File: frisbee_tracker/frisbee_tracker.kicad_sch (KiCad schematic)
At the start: 18 parts, among them IC1 NRF54L05-QFAA-R7, J1 UJC-H-G-SMT-2-P6-TR, U1 AP2210N-3.3TRG1, U2 BQ24072RGTT, U3 BMI323

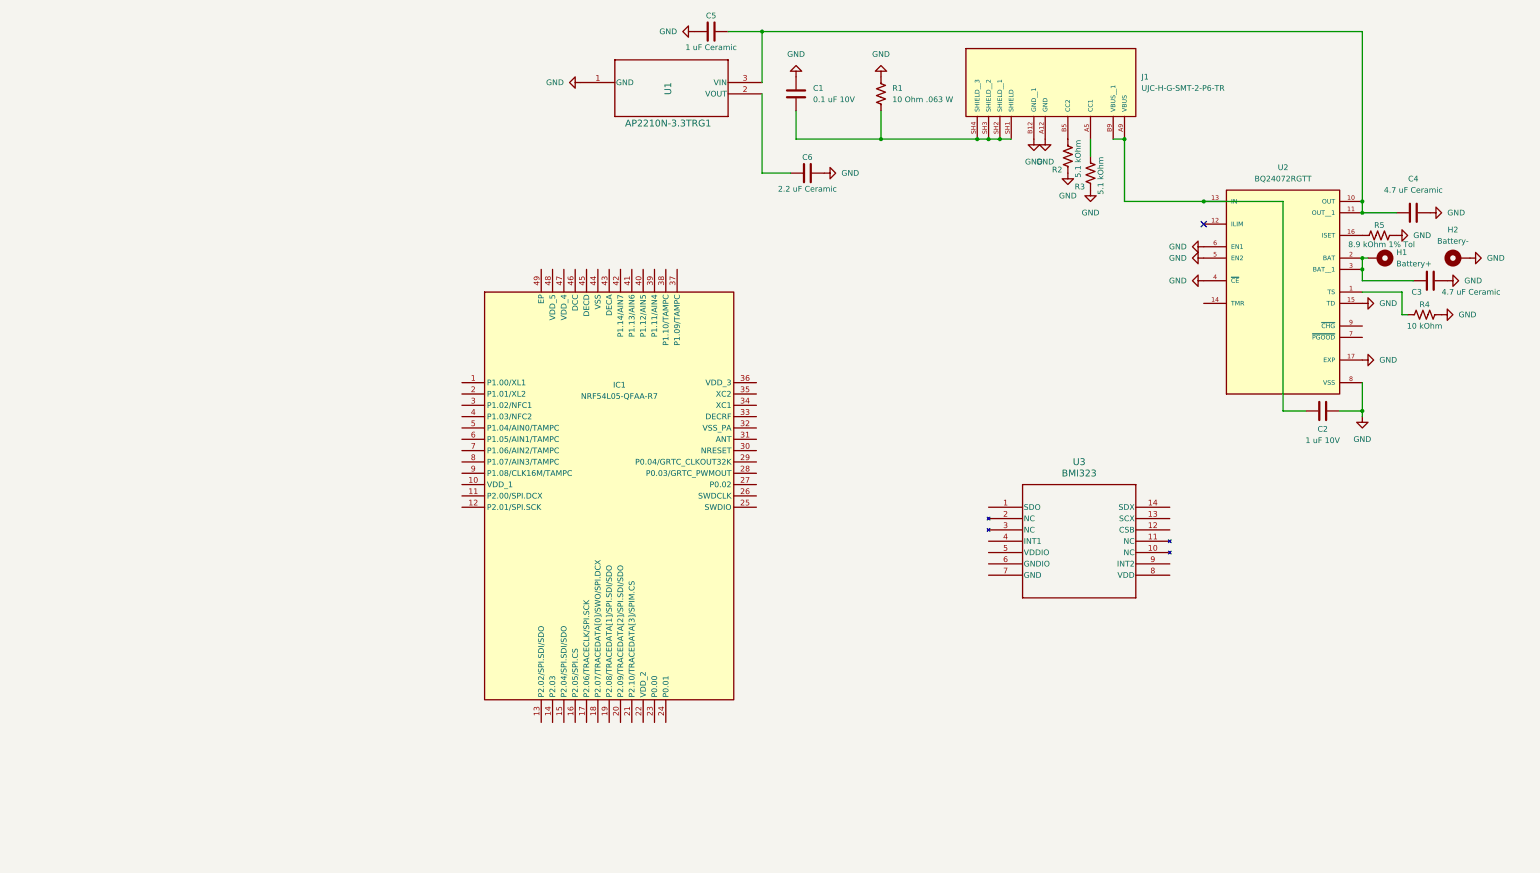
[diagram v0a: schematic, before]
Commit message: Rough draft of schematic complete
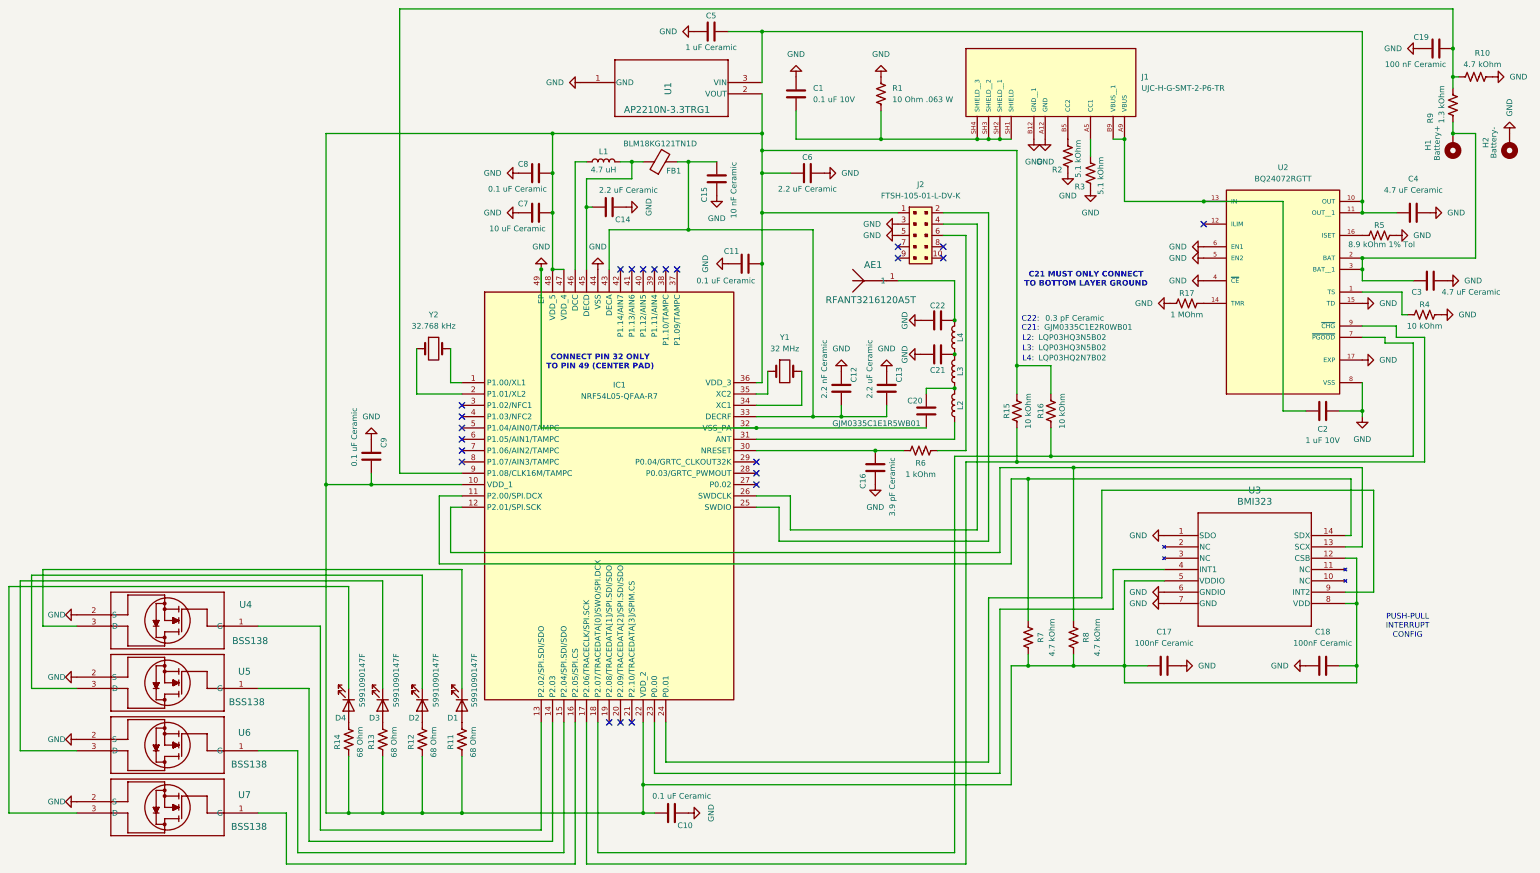
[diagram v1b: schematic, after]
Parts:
- added AE1: RFANT3216120A5T, ANT_RFANT3216120A5T_WAL, symbol RFANT3216120A5T:RFANT3216120A5T
- added C10, C11, C8, C9: 0.1 uF Ceramic, symbol Device:C
- added C12: 2.2 nF Ceramic, symbol Device:C
- added C13, C14: 2.2 uF Ceramic, symbol Device:C
- added C15: 10 nF Ceramic, symbol Device:C
- added C16: 3.9 pF Ceramic, symbol Device:C
- added C17, C18: 100nF Ceramic, symbol Device:C
- added C19: 100 nF Ceramic, symbol Device:C
- added C20: GJM0335C1E1R5WB01, symbol Device:C
- added C21: GJM0335C1E2R0WB01, symbol Device:C
- added C22: 0.3 pF Ceramic, symbol Device:C
- added C7: 10 uF Ceramic, symbol Device:C
- added D1, D2, D3, D4: 5991090147F, symbol Device:LED
- added FB1: BLM18KG121TN1D, symbol Device:FerriteBead
- added J2: FTSH-105-01-L-DV-K, digikey-footprints:PinHeader_2x5_P1.27_SMD, symbol dk_Rectangular-Connectors-Headers-Male-Pins:FTSH-105-01-L-DV-K
- added L1: 4.7 uH, symbol Device:L
- added L2: LQP03HQ2N7B02, symbol Device:L
- added L3, L4: LQP03HQ3N5B02, symbol Device:L
- added R10, R7, R8: 4.7 kOhm, symbol Device:R_US
- added R11, R12, R13, R14: 68 Ohm, symbol Device:R_US
- added R15, R16: 10 kOhm, symbol Device:R_US
- added R17: 1 MOhm, symbol Device:R_US
- added R6: 1 kOhm, symbol Device:R_US
- added R9: 1.3 kOhm, symbol Device:R_US
- added U4, U5, U6, U7: BSS138, SOT-23_3L_ONS, symbol BSS138:BSS138
- added Y1: 32 MHz, symbol Device:Crystal
- added Y2: 32.768 kHz, symbol Device:Crystal
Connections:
- net GND: now also IC1.32 (VSS_PA), IC1.44 (VSS), IC1.49 (EP), U3.1 (SDO), U3.6 (GNDIO), U3.7 (GND), C10.1, C11.1, C12.1, C13.1, C14.1, C15.1, C16.1, C17.2, C18.1, C19.1, C20.1, C21.2, C22.1, C7.1, C8.1, C9.1, J2.3, J2.5, R10.2, R17.1, U4.2 (S), U5.2 (S), U6.2 (S), U7.2 (S)
- net at U2.14 (TMR): now also R17.2
- net at C3.1, H1.1, U2.2 (BAT)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: now also R9.2
- net at U2.7 (~{PGOOD}): now also IC1.18 (P2.07/TRACEDATA[0]/SWO/SPI.DCX), R16.1
- net at U2.9 (~{CHG}): now also IC1.17 (P2.06/TRACECLK/SPI.SCK), R15.1
- net at C6.1, U1.2 (VOUT): now also IC1.10 (VDD_1), IC1.22 (VDD_2), IC1.36 (VDD_3), IC1.47 (VDD_4), IC1.48 (VDD_5), U3.12 (CSB), U3.5 (VDDIO), U3.8 (VDD), C10.2, C11.2, C17.1, C18.2, C7.2, C8.2, C9.2, J2.1, R11.2, R12.2, R13.2, R14.2, R15.2, R16.2, R7.1, R8.1
- net at U3.13 (SCX): now also IC1.12 (P2.01/SPI.SCK), R8.2
- net at U3.14 (SDX): now also IC1.11 (P2.00/SPI.DCX), R7.2
- net at U3.4 (INT1): now also IC1.23 (P0.00)
- net at U3.9 (INT2): now also IC1.24 (P0.01)
- net at IC1.1 (P1.00/XL1): now also Y2.2
- net at IC1.13 (P2.02/SPI.SDI/SDO): now also U4.1 (G)
- net at IC1.14 (P2.03): now also U5.1 (G)
- net at IC1.15 (P2.04/SPI.SDI/SDO): now also U6.1 (G)
- net at IC1.16 (P2.05/SPI.CS): now also U7.1 (G)
- net at IC1.2 (P1.01/XL2): now also Y2.1
- net at IC1.25 (SWDIO): now also J2.2
- net at IC1.26 (SWDCLK): now also J2.4
- net at IC1.30 (NRESET): now also C16.2, R6.1
- net at IC1.31 (ANT): now also L2.1
- net at IC1.33 (DECRF): now also IC1.43 (DECA), C12.2, C13.2, C15.2, FB1.2
- net at IC1.34 (XC1): now also Y1.2
- net at IC1.35 (XC2): now also Y1.1
- net at IC1.45 (DECD): now also C14.2, FB1.1, L1.2
- net at IC1.46 (DCC): now also L1.1
- net at IC1.9 (P1.08/CLK16M/TAMPC): now also C19.2, R10.1, R9.1
- new net: D4.2 (A), R14.1
- new net: D2.1 (K), U5.3 (D)
- new net: D2.2 (A), R12.1
- new net: D3.2 (A), R13.1
- new net: D3.1 (K), U6.3 (D)
- new net: D1.1 (K), U4.3 (D)
- new net: D1.2 (A), R11.1
- new net: C20.2, L2.2, L3.1
- new net: C21.1, L3.2, L4.1
- new net: J2.6, R6.2
- new net: D4.1 (K), U7.3 (D)
- new net: AE1.1, C22.2, L4.2
- no-connect marks 1 -> 23
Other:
- note added: "C21 MUST ONLY CONNECT TO BOTTOM LAYER GROUND"
- note added: "C21:"
- note added: "C22:"
- note added: "CONNECT PIN 32 ONLY TO PIN 49 (CENTER PAD)"
- note added: "L2:"
- note added: "L3:"
- note added: "L4:"
- note added: "PUSH-PULL INTERRUPT CONFIG"
- moved on the sheet: H1, H2, U3

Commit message: start of PCB design
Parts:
- AE1: footprint ANT_RFANT3216120A5T_WAL -> footprints:RFANT3216120A5T
- C1, C10, C11, C12, C13, C14, C15, C16, C17, C18, C19, C2, C22, C3, C4, C5, C6, C7, C8, C9: footprint (none) -> Capacitor_SMD:C_0603_1608Metric
- C20, C21: footprint (none) -> Capacitor_SMD:C_0201_0603Metric
- D1, D2, D3, D4: footprint (none) -> LED_SMD:LED_0603_1608Metric
- FB1: footprint (none) -> footprints:BLM18KG121TN1D
- H1, H2: footprint (none) -> Connector_PinHeader_1.27mm:PinHeader_1x01_P1.27mm_Vertical
- IC1: footprint (none) -> footprints:NRF54L05-QFAA-R7
- J1: footprint (none) -> footprints:UJC-H-G-SMT-2-P6-TR
- J2: footprint digikey-footprints:PinHeader_2x5_P1.27_SMD -> footprints:FTSH-105-01-L-DV-K
- L1: footprint (none) -> Inductor_SMD:L_0603_1608Metric
- L2: footprint (none) -> footprints:LQP03HQ2N7B02D
- L3, L4: footprint (none) -> footprints:LQP03HQ3N5B02D
- R1, R10, R11, R12, R13, R14, R15, R16, R17, R2, R3, R4, R5, R6, R7, R8, R9: footprint (none) -> Resistor_SMD:R_0603_1608Metric
- U1: footprint (none) -> footprints:AP2210N-3.3TRG1
- U2: footprint (none) -> footprints:BQ24072RGTT
- U3: footprint (none) -> footprints:BMI323
- U4, U5, U6, U7: footprint SOT-23_3L_ONS -> footprints:BSS138
- Y1: footprint (none) -> footprints:ECS-320-8-37B2-JTY-TR
- Y2: footprint (none) -> footprints:Q 0,032768-JTX210-7-20-T1-HMR-70K-LF
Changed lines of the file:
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@@
 			)
 		)
-		(property "Footprint" ""
+		(property "Footprint" "footprints:Q 0,032768-JTX210-7-20-T1-HMR-70K-LF"
 			(at 38.1 88.9 0)
 			(effects
@@
 			)
 		)
-		(property "Footprint" ""
+		(property "Footprint" "Capacitor_SMD:C_0603_1608Metric"
 			(at 120.3452 35.56 0)
 			(effects
@@
 			)
 		)
-		(property "Footprint" ""
+		(property "Footprint" "Capacitor_SMD:C_0603_1608Metric"
 			(at 241.3 101.9048 0)
 			(effects
@@
 			)
 		)
-		(property "Footprint" ""
+		(property "Footprint" "Capacitor_SMD:C_0603_1608Metric"
 			(at 73.66 58.1152 0)
 			(effects
@@
 			)
 		)
-		(property "Footprint" ""
+		(property "Footprint" "Resistor_SMD:R_0603_1608Metric"
 			(at 20.066 176.784 90)
 			(effects
@@
 			)
 		)
-		(property "Footprint" ""
+		(property "Footprint" "LED_SMD:LED_0603_1608Metric"
 			(at 35.56 168.91 0)
 			(effects
@@
 			)
 		)
-		(property "Footprint" ""
+		(property "Footprint" "Resistor_SMD:R_0603_1608Metric"
 			(at 27.686 176.784 90)
 			(effects
@@
 			)
 		)
-		(property "Footprint" ""
+		(property "Footprint" "LED_SMD:LED_0603_1608Metric"
 			(at 26.67 168.91 0)
 			(effects
@@
 			)
 		)
-		(property "Footprint" ""
+		(property "Footprint" "Capacitor_SMD:C_0603_1608Metric"
 			(at 100.6348 46.99 0)
 			(effects
@@
 			)
 		)
-		(property "Footprint" ""
+		(property "Footprint" "Capacitor_SMD:C_0603_1608Metric"
 			(at 25.0952 116.84 0)
 			(effects
@@
 			)
 		)
-		(property "Footprint" ""
+		(property "Footprint" "footprints:BQ24072RGTT"
 			(at 228.6 73.66 0)
 			(effects
@@
 			)
 		)
-		(property "Footprint" ""
+		(property "Footprint" "Resistor_SMD:R_0603_1608Metric"
 			(at 181.356 45.974 90)
 			(effects
@@
 			)
 		)
-		(property "Footprint" "SOT-23_3L_ONS"
+		(property "Footprint" "footprints:BSS138"
 			(at -1.27 151.13 0)
 			(effects
@@
 			)
 		)
-		(property "Footprint" ""
+		(property "Footprint" "Capacitor_SMD:C_0603_1608Metric"
 			(at 261.62 57.4548 0)
 			(effects
@@
 			)
 		)
-		(property "Footprint" ""
+		(property "Footprint" "Resistor_SMD:R_0603_1608Metric"
 			(at 45.466 176.784 90)
 			(effects
@@
 			)
 		)
-		(property "Footprint" ""
+		(property "Footprint" "Resistor_SMD:R_0603_1608Metric"
 			(at 260.604 80.264 90)
 			(effects
@@
 			)
 		)
-		(property "Footprint" ""
+		(property "Footprint" "Capacitor_SMD:C_0603_1608Metric"
 			(at 265.43 72.6948 0)
 			(effects
@@
 			)
 		)
-		(property "Footprint" ""
+		(property "Footprint" "Capacitor_SMD:C_0603_1608Metric"
 			(at 125.73 48.5648 0)
 			(effects
@@
 			)
 		)
-		(property "Footprint" ""
+		(property "Footprint" "Resistor_SMD:R_0603_1608Metric"
 			(at 175.514 102.616 90)
 			(effects
@@
 			)
 		)
-		(property "Footprint" ""
+		(property "Footprint" "Resistor_SMD:R_0603_1608Metric"
 			(at 186.436 49.784 90)
 			(effects
@@
 			)
 		)
-		(property "Footprint" ""
+		(property "Footprint" "Capacitor_SMD:C_0603_1608Metric"
 			(at 266.7 20.6248 0)
 			(effects
@@
 			)
 		)
-		(property "Footprint" ""
+		(property "Footprint" "Connector_PinHeader_1.27mm:PinHeader_1x01_P1.27mm_Vertical"
 			(at 266.7 43.18 0)
 			(effects
@@
 			)
 		)
-		(property "Footprint" "SOT-23_3L_ONS"
+		(property "Footprint" "footprints:BSS138"
 			(at -1.27 179.07 0)
 			(effects
@@
 			)
 		)
-		(property "Footprint" ""
+		(property "Footprint" "footprints:LQP03HQ3N5B02D"
 			(at 154.94 93.98 0)
 			(effects
@@
 			)
 		)
-		(property "Footprint" ""
+		(property "Footprint" "Resistor_SMD:R_0603_1608Metric"
 			(at 167.894 102.616 90)
 			(effects
@@
 			)
 		)
-		(property "Footprint" ""
+		(property "Footprint" "footprints:BMI323"
 			(at 201.93 130.81 0)
 			(effects
@@
 			)
 		)
-		(property "Footprint" ""
+		(property "Footprint" "Resistor_SMD:R_0603_1608Metric"
 			(at 272.034 26.924 90)
 			(effects
@@
 			)
 		)
-		(property "Footprint" ""
+		(property "Footprint" "footprints:BLM18KG121TN1D"
 			(at 88.9 48.768 90)
 			(effects
@@
 			)
 		)
-		(property "Footprint" ""
+		(property "Footprint" "Resistor_SMD:R_0603_1608Metric"
 			(at 147.574 110.744 90)
 			(effects
@@
 			)
 		)
-		(property "Footprint" ""
+		(property "Footprint" "Capacitor_SMD:C_0603_1608Metric"
 			(at 130.5052 101.6 0)
 			(effects
@@
 			)
 		)
-		(property "Footprint" ""
+		(property "Footprint" "Capacitor_SMD:C_0603_1608Metric"
 			(at 64.77 57.4548 0)
 			(effects
@@
 			)
 		)
-		(property "Footprint" "SOT-23_3L_ONS"
+		(property "Footprint" "footprints:BSS138"
 			(at -1.27 193.04 0)
 			(effects
@@
 			)
 		)
-		(property "Footprint" ""
+		(property "Footprint" "Resistor_SMD:R_0603_1608Metric"
 			(at 139.446 32.004 90)
 			(effects
@@
 			)
 		)
-		(property "Footprint" ""
+		(property "Footprint" "Capacitor_SMD:C_0603_1608Metric"
 			(at 205.74 159.0548 0)
 			(effects
@@
 			)
 		)
-		(property "Footprint" "SOT-23_3L_ONS"
+		(property "Footprint" "footprints:BSS138"
 			(at -1.27 165.1 0)
 			(effects
@@
 			)
 		)
-		(property "Footprint" ""
+		(property "Footprint" "Resistor_SMD:R_0603_1608Metric"
 			(at 207.264 77.724 90)
 			(effects
@@
 			)
 		)
-		(property "Footprint" ""
+		(property "Footprint" "Capacitor_SMD:C_0603_1608Metric"
 			(at 64.77 48.5648 0)
 			(effects
@@
 			)
 		)
-		(property "Footprint" ""
+		(property "Footprint" "Capacitor_SMD:C_0603_1608Metric"
 			(at 87.63 194.0052 0)
 			(effects
@@
 			)
 		)
-		(property "Footprint" ""
+		(property "Footprint" "Capacitor_SMD:C_0201_0603Metric"
 			(at 147.32 91.1352 0)
 			(effects
@@
 			)
 		)
-		(property "Footprint" ""
+		(property "Footprint" "Resistor_SMD:R_0603_1608Metric"
 			(at 250.444 62.484 90)
 			(effects
@@
 			)
 		)
-		(property "Footprint" ""
+		(property "Footprint" "Capacitor_SMD:C_0603_1608Metric"
 			(at 154.94 81.5848 0)
 			(effects
@@
 			)
 		)
-		(property "Footprint" ""
+		(property "Footprint" "footprints:UJC-H-G-SMT-2-P6-TR"
 			(at 182.88 29.21 0)
 			(effects
@@
 			)
 		)
-		(property "Footprint" ""
+		(property "Footprint" "Capacitor_SMD:C_0603_1608Metric"
 			(at 140.6652 101.6 0)
 			(effects
@@
 			)
 		)
-		(property "Footprint" "ANT_RFANT3216120A5T_WAL"
+		(property "Footprint" "footprints:RFANT3216120A5T"
 			(at 142.24 73.66 0)
 			(effects
@@
 			)
 		)
-		(property "Footprint" ""
+		(property "Footprint" "footprints:ECS-320-8-37B2-JTY-TR"
 			(at 116.84 93.98 0)
 			(effects
@@
 			)
 		)
-		(property "Footprint" ""
+		(property "Footprint" "LED_SMD:LED_0603_1608Metric"
 			(at 44.45 168.91 0)
 			(effects
@@
 			)
 		)
-		(property "Footprint" ""
+		(property "Footprint" "Capacitor_SMD:C_0201_0603Metric"
 			(at 147.6248 99.06 0)
 			(effects
@@
 			)
 		)
-		(property "Footprint" ""
+		(property "Footprint" "footprints:LQP03HQ3N5B02D"
 			(at 154.94 86.36 0)
 			(effects
@@
 			)
 		)
-		(property "Footprint" ""
+		(property "Footprint" "LED_SMD:LED_0603_1608Metric"
 			(at 19.05 168.91 0)
 			(effects
@@
 			)
 		)
-		(property "Footprint" ""
+		(property "Footprint" "footprints:NRF54L05-QFAA-R7"
 			(at 106.68 173.66 0)
 			(effects
@@
 			)
 		)
-		(property "Footprint" ""
+		(property "Footprint" "Capacitor_SMD:C_0603_1608Metric"
 			(at 104.14 16.8148 0)
 			(effects
@@
 			)
 		)
-		(property "Footprint" ""
+		(property "Footprint" "Capacitor_SMD:C_0603_1608Metric"
 			(at 111.76 68.8848 0)
 			(effects
@@
 			)
 		)
-		(property "Footprint" ""
+		(property "Footprint" "Resistor_SMD:R_0603_1608Metric"
 			(at 36.576 176.784 90)
 			(effects
@@
 			)
 		)
-		(property "Footprint" ""
+		(property "Footprint" "footprints:LQP03HQ2N7B02D"
 			(at 154.94 101.6 0)
 			(effects
@@
 			)
 		)
-		(property "Footprint" ""
+		(property "Footprint" "Resistor_SMD:R_0603_1608Metric"
 			(at 170.434 153.416 90)
 			(effects
@@
 			)
 		)
-		(property "Footprint" ""
+		(property "Footprint" "Capacitor_SMD:C_0603_1608Metric"
 			(at 241.3 159.0548 0)
 			(effects
@@
 			)
 		)
-		(property "Footprint" ""
+		(property "Footprint" "Inductor_SMD:L_0603_1608Metric"
 			(at 76.2 46.99 0)
 			(effects
@@
 			)
 		)
-		(property "Footprint" "digikey-footprints:PinHeader_2x5_P1.27_SMD"
+		(property "Footprint" "footprints:FTSH-105-01-L-DV-K"
 			(at 152.4 58.42 0)
 			(effects
@@
 			)
 		)
-		(property "Footprint" ""
+		(property "Footprint" "Connector_PinHeader_1.27mm:PinHeader_1x01_P1.27mm_Vertical"
 			(at 279.4 43.18 0)
 			(effects
@@
 			)
 		)
-		(property "Footprint" ""
+		(property "Footprint" "Resistor_SMD:R_0603_1608Metric"
 			(at 180.594 153.416 90)
 			(effects
@@
 			)
 		)
-		(property "Footprint" ""
+		(property "Footprint" "Resistor_SMD:R_0603_1608Metric"
 			(at 267.716 34.544 90)
 			(effects
@@
 			)
 		)
-		(property "Footprint" ""
+		(property "Footprint" "footprints:AP2210N-3.3TRG1"
 			(at 71.12 29.21 0)
 			(effects
@@
 			)
 		)
-		(property "Footprint" ""
+		(property "Footprint" "Capacitor_SMD:C_0603_1608Metric"
 			(at 136.1948 111.76 0)
 			(effects
